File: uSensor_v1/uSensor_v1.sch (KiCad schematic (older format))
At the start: 224 parts, among them J1 +12V Supply, J2 Conn_01x03, J3 Conn_01x03, J4 NS25-W8P 6-pin 2,54mm, J5 USB_B, J6 GNDA-GNDD Jumper, J7 Barrel_Jack_Switch, Q1 BC817-25, Q2 BC817-25, SW1 SW_Push, SW2 SW_Push, SW3 SW_Push, U1 AM10TW-2405DZ, U10 KSS-213 Connector, U11 AD7795, U12 AD5667, U13 TBD, U15 REF192, U2 LD1117A, U22 RCLAMP, U3 STM32F407VGTx, U4 MCP9700AT, U5 MCP9700AT, U6 LM6132A, U7 MCP9700AT, U8 MCP9700AT, U9 UG-2864KSWLG01

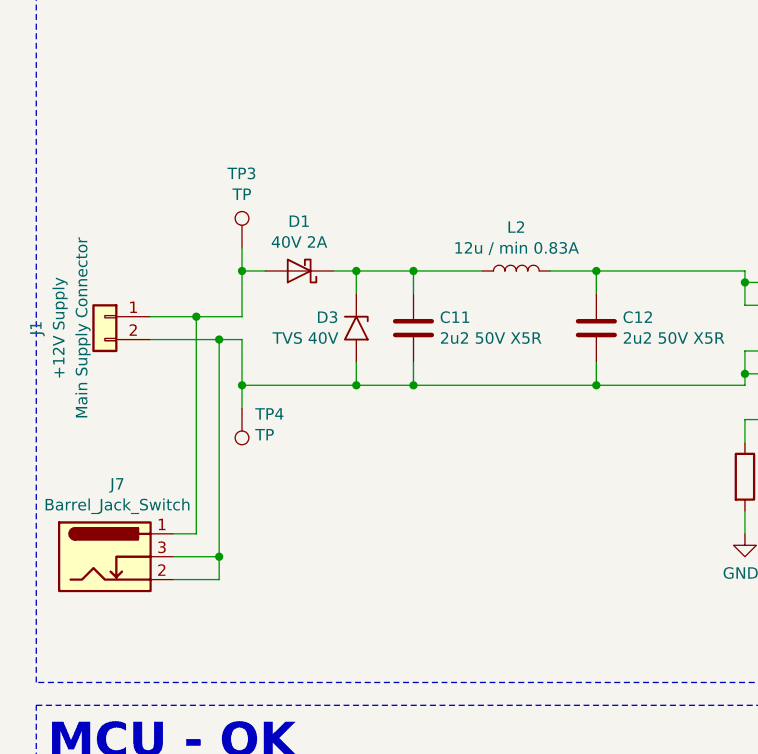
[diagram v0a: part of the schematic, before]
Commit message: Layout ready to 1st review.
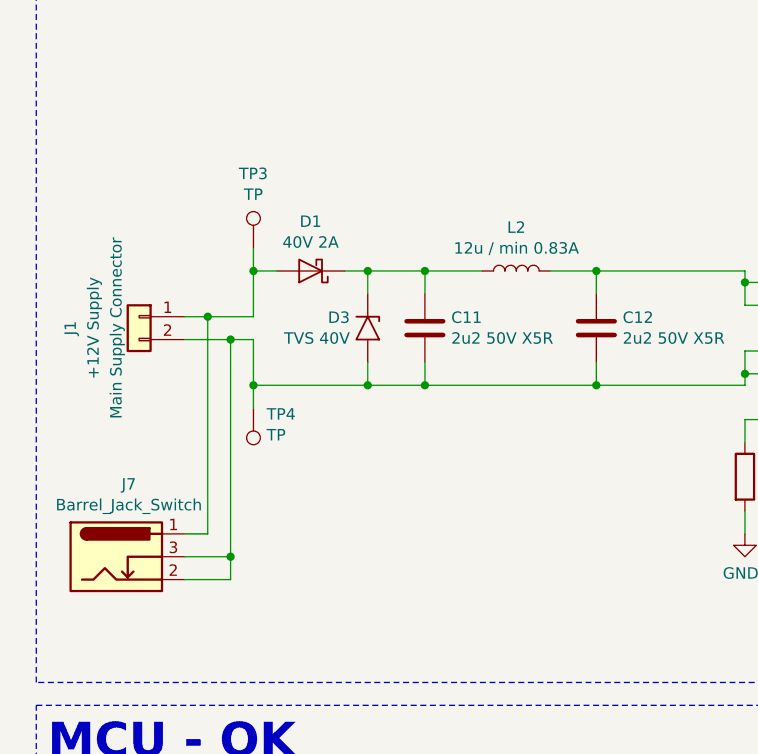
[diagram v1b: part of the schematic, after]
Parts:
- J1: footprint Connector_PinHeader_2.54mm:PinHeader_1x02_P2.54mm_Vertical -> Connector_Molex:Molex_KK-254_AE-6410-02A_1x02_P2.54mm_Vertical
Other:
- moved on the sheet: C11, D1, D3, J1, J7, TP3, TP4
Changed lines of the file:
@@
 L Connector_Generic:Conn_01x02 J1
 U 1 1 5C42724A
-P 850 2200
-F 0 "J1" V 1150 2150 50  0000 C CNN
-F 1 "+12V Supply" V 1050 2150 50  0000 C CNN
-F 2 "Connector_PinHeader_2.54mm:PinHeader_1x02_P2.54mm_Vertical" H 850 2200 50  0001 C CNN
-F 3 "~" H 850 2200 50  0001 C CNN
-F 4 "Main Supply Connector" V 950 2150 50  0000 C CNN "Function"
-	1    850  2200
+P 1000 2200
+F 0 "J1" V 1300 2150 50  0000 C CNN
+F 1 "+12V Supply" V 1200 2150 50  0000 C CNN
+F 2 "Connector_Molex:Molex_KK-254_AE-6410-02A_1x02_P2.54mm_Vertical" H 1000 2200 50  0001 C CNN
+F 3 "~" H 1000 2200 50  0001 C CNN
+F 4 "Main Supply Connector" V 1100 2150 50  0000 C CNN "Function"
+	1    1000 2200
 	-1   0    0    -1
 $EndComp
@@
 L Device:C C11
 U 1 1 5C427492
-P 2200 2250
-F 0 "C11" H 2315 2296 50  0000 L CNN
-F 1 "2u2 50V X5R" H 2315 2205 50  0000 L CNN
-F 2 "Resistor_SMD:R_0805_2012Metric_Pad1.15x1.40mm_HandSolder" H 2238 2100 50  0001 C CNN
-F 3 "~" H 2200 2250 50  0001 C CNN
-	1    2200 2250
+P 2250 2250
+F 0 "C11" H 2365 2296 50  0000 L CNN
+F 1 "2u2 50V X5R" H 2365 2205 50  0000 L CNN
+F 2 "Resistor_SMD:R_0805_2012Metric_Pad1.15x1.40mm_HandSolder" H 2288 2100 50  0001 C CNN
+F 3 "~" H 2250 2250 50  0001 C CNN
+	1    2250 2250
 	1    0    0    -1
 $EndComp
@@
 	3000 2500 3000 2400
 Wire Wire Line
-	2200 2500 2200 2400
+	2250 2500 2250 2400
 Wire Wire Line
-	1050 2300 1350 2300
+	1200 2300 1400 2300
 Wire Wire Line
-	1450 2300 1450 2500
-Connection ~ 2200 2500
+	1500 2300 1500 2500
+Connection ~ 2250 2500
 Wire Wire Line
-	1050 2200 1250 2200
+	1200 2200 1300 2200
 Wire Wire Line
-	1450 2200 1450 2000
+	1500 2200 1500 2000
 Wire Wire Line
-	2200 2000 2200 2100
+	2250 2000 2250 2100
 Wire Wire Line
-	2500 2000 2200 2000
+	2500 2000 2250 2000
 Wire Wire Line
 	2800 2000 3000 2000
@@
 L Device:D_Schottky D1
 U 1 1 5CAE2AA1
-P 1700 2000
-F 0 "D1" H 1700 1784 50  0000 C CNN
-F 1 "40V 2A" H 1700 1875 50  0000 C CNN
-F 2 "Sentisa-Diodes:D_SMB" H 1700 2000 50  0001 C CNN
-F 3 "~" H 1700 2000 50  0001 C CNN
-F 4 "Diotec Semiconductor" H 1700 2000 50  0001 C CNN "MFR"
-F 5 "SK25" H 1700 2000 50  0001 C CNN "MPN"
-	1    1700 2000
+P 1750 2000
+F 0 "D1" H 1750 1784 50  0000 C CNN
+F 1 "40V 2A" H 1750 1875 50  0000 C CNN
+F 2 "Sentisa-Diodes:D_SMB" H 1750 2000 50  0001 C CNN
+F 3 "~" H 1750 2000 50  0001 C CNN
+F 4 "Diotec Semiconductor" H 1750 2000 50  0001 C CNN "MFR"
+F 5 "SK25" H 1750 2000 50  0001 C CNN "MPN"
+	1    1750 2000
 	-1   0    0    1
 $EndComp
 Wire Wire Line
-	1850 2000 1950 2000
-Connection ~ 2200 2000
+	1900 2000 2000 2000
+Connection ~ 2250 2000
 $Comp
 L Device:R R6
@@
 L Diode:1.5KExxA D3
 U 1 1 5E6A365E
-P 1950 2250
-F 0 "D3" V 1904 2172 50  0000 R CNN
-F 1 "TVS 40V" V 1995 2172 50  0000 R CNN
-F 2 "Sentisa-Diodes:D_SMB" H 1950 2050 50  0001 C CNN
-F 3 "" H 1900 2250 50  0001 C CNN
-F 4 "Vishay" V 1950 2250 50  0001 C CNN "MPN"
-F 5 "SMBJ40D-M3/H" V 1950 2250 50  0001 C CNN "MFR"
-	1    1950 2250
+P 2000 2250
+F 0 "D3" V 1954 2172 50  0000 R CNN
+F 1 "TVS 40V" V 2045 2172 50  0000 R CNN
+F 2 "Sentisa-Diodes:D_SMB" H 2000 2050 50  0001 C CNN
+F 3 "" H 1950 2250 50  0001 C CNN
+F 4 "Vishay" V 2000 2250 50  0001 C CNN "MPN"
+F 5 "SMBJ40D-M3/H" V 2000 2250 50  0001 C CNN "MFR"
+	1    2000 2250
 	0    1    1    0
 $EndComp
 Wire Wire Line
-	1450 2000 1550 2000
+	1500 2000 1600 2000
 Wire Wire Line
-	1450 2500 1950 2500
+	1500 2500 2000 2500
 Wire Wire Line
-	1950 2100 1950 2000
-Connection ~ 1950 2000
+	2000 2100 2000 2000
+Connection ~ 2000 2000
 Wire Wire Line
-	1950 2000 2200 2000
+	2000 2000 2250 2000
 Wire Wire Line
-	1950 2400 1950 2500
-Connection ~ 1950 2500
+	2000 2400 2000 2500
+Connection ~ 2000 2500
 Text GLabel 8400 14650 2    50   Output ~ 0
 DAC_OUT_COIL_T_CTRL
 Wire Wire Line
-	1950 2500 2200 2500
+	2000 2500 2250 2500
 Wire Wire Line
-	2200 2500 3000 2500
+	2250 2500 3000 2500
 Wire Wire Line
 	20750 5550 20950 5550
@@
 L Connector:TestPoint TP3
 U 1 1 5C3E6779
-P 1450 1900
-F 0 "TP3" H 1450 2225 50  0000 C CNN
-F 1 "TP" H 1450 2134 50  0000 C CNN
-F 2 "Sentisa-Connectors:TestPoint_Probe_1.0mmDiameter_0.6mmDrill" H 1650 1900 50  0001 C CNN
-F 3 "~" H 1650 1900 50  0001 C CNN
-	1    1450 1900
+P 1500 1900
+F 0 "TP3" H 1500 2225 50  0000 C CNN
+F 1 "TP" H 1500 2134 50  0000 C CNN
+F 2 "Sentisa-Connectors:TestPoint_Probe_1.0mmDiameter_0.6mmDrill" H 1700 1900 50  0001 C CNN
+F 3 "~" H 1700 1900 50  0001 C CNN
+	1    1500 1900
 	1    0    0    -1
 $EndComp
@@
 L Connector:TestPoint TP4
 U 1 1 5C459570
-P 1450 2600
-F 0 "TP4" H 1392 2627 50  0000 R CNN
-F 1 "TP" H 1392 2718 50  0000 R CNN
-F 2 "Sentisa-Connectors:TestPoint_Probe_1.0mmDiameter_0.6mmDrill" H 1650 2600 50  0001 C CNN
-F 3 "~" H 1650 2600 50  0001 C CNN
-	1    1450 2600
+P 1500 2600
+F 0 "TP4" H 1442 2627 50  0000 R CNN
+F 1 "TP" H 1442 2718 50  0000 R CNN
+F 2 "Sentisa-Connectors:TestPoint_Probe_1.0mmDiameter_0.6mmDrill" H 1700 2600 50  0001 C CNN
+F 3 "~" H 1700 2600 50  0001 C CNN
+	1    1500 2600
 	-1   0    0    1
 $EndComp
@@
 	9700 24550 9800 24550
 Wire Wire Line
-	1450 2600 1450 2500
-Connection ~ 1450 2500
+	1500 2600 1500 2500
+Connection ~ 1500 2500
 Wire Wire Line
-	1450 1900 1450 2000
-Connection ~ 1450 2000
+	1500 1900 1500 2000
+Connection ~ 1500 2000
 Wire Wire Line
 	7000 1650 7000 1750
@@
 L Connector:Barrel_Jack_Switch J7
 U 1 1 5CBD7599
-P 850 3250
-F 0 "J7" H 905 3567 50  0000 C CNN
-F 1 "Barrel_Jack_Switch" H 905 3476 50  0000 C CNN
-F 2 "Connector_BarrelJack:BarrelJack_Wuerth_6941xx301002" H 900 3210 50  0001 C CNN
-F 3 "~" H 900 3210 50  0001 C CNN
-	1    850  3250
+P 900 3250
+F 0 "J7" H 955 3567 50  0000 C CNN
+F 1 "Barrel_Jack_Switch" H 955 3476 50  0000 C CNN
+F 2 "Connector_BarrelJack:BarrelJack_Wuerth_6941xx301002" H 950 3210 50  0001 C CNN
+F 3 "~" H 950 3210 50  0001 C CNN
+	1    900  3250
 	1    0    0    -1
 $EndComp
 Wire Wire Line
-	1150 3150 1250 3150
+	1200 3150 1300 3150
 Wire Wire Line
-	1250 3150 1250 2200
-Connection ~ 1250 2200
+	1300 3150 1300 2200
+Connection ~ 1300 2200
 Wire Wire Line
-	1250 2200 1450 2200
+	1300 2200 1500 2200
 Wire Wire Line
-	1150 3250 1350 3250
+	1200 3250 1400 3250
 Wire Wire Line
-	1350 3250 1350 2300
-Connection ~ 1350 2300
+	1400 3250 1400 2300
+Connection ~ 1400 2300
 Wire Wire Line
-	1350 2300 1450 2300
+	1400 2300 1500 2300
 Wire Wire Line
-	1150 3350 1350 3350
+	1200 3350 1400 3350
 Wire Wire Line
-	1350 3350 1350 3250
-Connection ~ 1350 3250
+	1400 3350 1400 3250
+Connection ~ 1400 3250
 Wire Wire Line
 	2600 18500 3700 18500
